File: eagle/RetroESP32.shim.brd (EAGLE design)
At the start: 56 x 34 mm, 2 parts

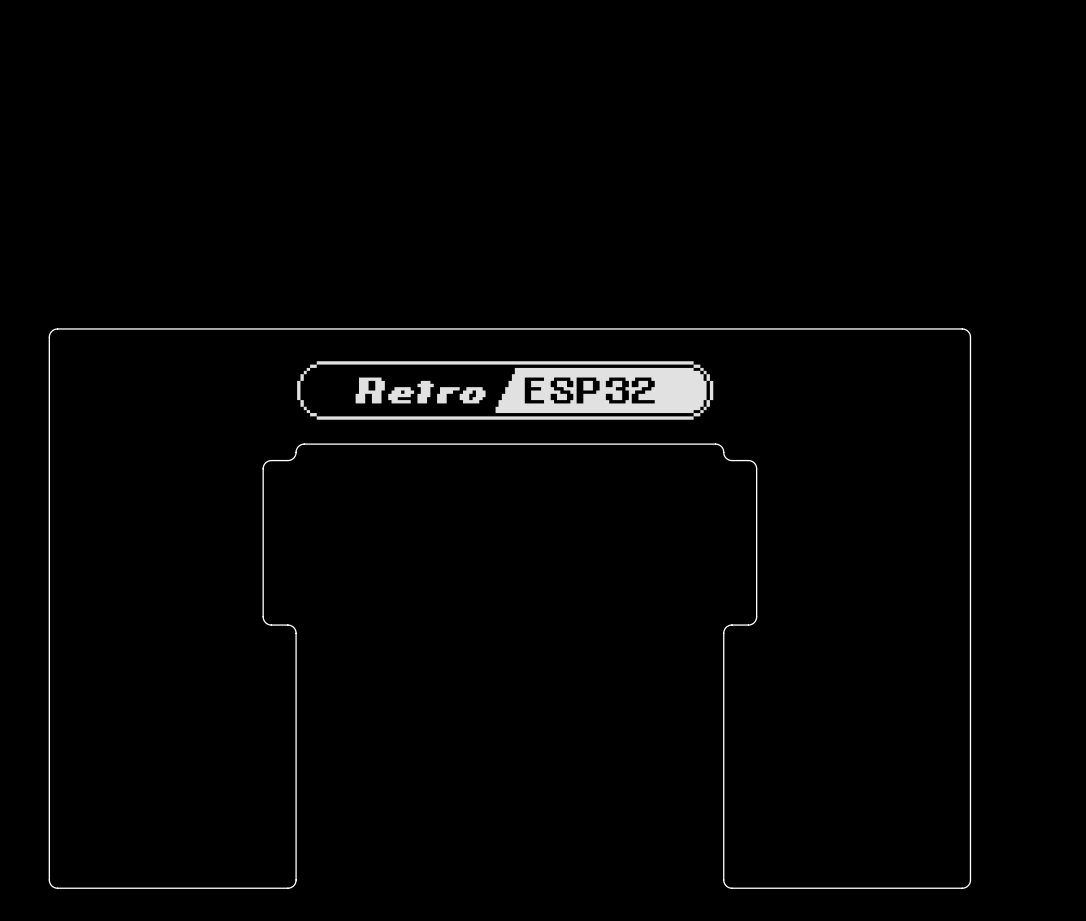
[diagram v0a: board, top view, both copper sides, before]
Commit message: feat: updated shim
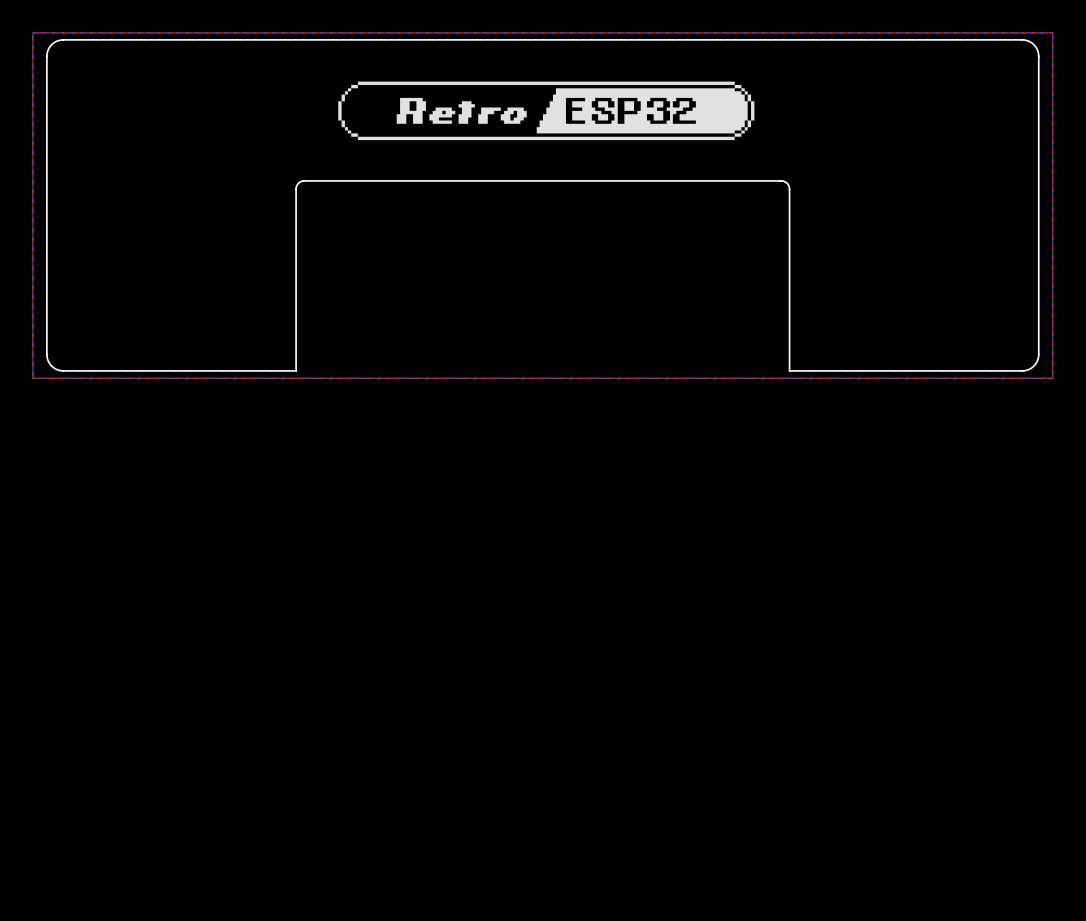
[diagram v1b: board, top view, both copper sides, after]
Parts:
- moved E$1 17.2 mm to (17.5, 49.0)
- moved U$1 17.1 mm to (38.5, 49.0)
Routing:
- added copper zone on layer 1, net GND
- added copper zone on layer 16, net GND
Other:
- board size 56 x 34 mm -> 60.3 x 20.1 mm
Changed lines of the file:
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@@
 <layer number="25" name="tNames" color="7" fill="1" visible="yes" active="yes"/>
 <layer number="26" name="bNames" color="7" fill="1" visible="yes" active="yes"/>
-<layer number="27" name="tValues" color="7" fill="1" visible="yes" active="yes"/>
-<layer number="28" name="bValues" color="7" fill="1" visible="yes" active="yes"/>
+<layer number="27" name="tValues" color="7" fill="1" visible="no" active="yes"/>
+<layer number="28" name="bValues" color="7" fill="1" visible="no" active="yes"/>
 <layer number="29" name="tStop" color="7" fill="3" visible="no" active="yes"/>
 <layer number="30" name="bStop" color="7" fill="6" visible="no" active="yes"/>
@@
 <layer number="41" name="tRestrict" color="4" fill="10" visible="yes" active="yes"/>
 <layer number="42" name="bRestrict" color="1" fill="10" visible="yes" active="yes"/>
-<layer number="43" name="vRestrict" color="2" fill="10" visible="yes" active="yes"/>
+<layer number="43" name="vRestrict" color="2" fill="10" visible="no" active="yes"/>
 <layer number="44" name="Drills" color="7" fill="1" visible="no" active="yes"/>
 <layer number="45" name="Holes" color="7" fill="1" visible="no" active="yes"/>
 <layer number="46" name="Milling" color="3" fill="1" visible="no" active="yes"/>
 <layer number="47" name="Measures" color="7" fill="1" visible="no" active="yes"/>
-<layer number="48" name="Document" color="7" fill="1" visible="yes" active="yes"/>
-<layer number="49" name="Reference" color="7" fill="1" visible="yes" active="yes"/>
+<layer number="48" name="Document" color="7" fill="1" visible="no" active="yes"/>
+<layer number="49" name="Reference" color="7" fill="1" visible="no" active="yes"/>
 <layer number="50" name="dxf" color="7" fill="1" visible="no" active="yes"/>
 <layer number="51" name="tDocu" color="7" fill="1" visible="yes" active="yes"/>
@@
 <board>
 <plain>
-<wire x1="0.5" y1="0" x2="14.5" y2="0" width="0" layer="20"/>
-<wire x1="14.5" y1="0" x2="15" y2="0.5" width="0" layer="20" curve="90"/>
-<wire x1="15" y1="0.5" x2="15" y2="15.5" width="0" layer="20"/>
-<wire x1="15" y1="15.5" x2="14.5" y2="16" width="0" layer="20" curve="90"/>
-<wire x1="15" y1="26.5" x2="15.5" y2="27" width="0" layer="20" curve="-90"/>
-<wire x1="15.5" y1="27" x2="40.5" y2="27" width="0" layer="20"/>
-<wire x1="40.5" y1="27" x2="41" y2="26.5" width="0" layer="20" curve="-90"/>
-<wire x1="41" y1="26.5" x2="41.5" y2="26" width="0" layer="20" curve="90"/>
-<wire x1="41.5" y1="26" x2="42.5" y2="26" width="0" layer="20"/>
-<wire x1="42.5" y1="26" x2="43" y2="25.5" width="0" layer="20" curve="-90"/>
-<wire x1="43" y1="25.5" x2="43" y2="16.5" width="0" layer="20"/>
-<wire x1="43" y1="16.5" x2="42.5" y2="16" width="0" layer="20" curve="-90"/>
-<wire x1="42.5" y1="16" x2="41.5" y2="16" width="0" layer="20"/>
-<wire x1="41.5" y1="16" x2="41" y2="15.5" width="0" layer="20" curve="90"/>
-<wire x1="41" y1="15.5" x2="41" y2="0.5" width="0" layer="20"/>
-<wire x1="41" y1="0.5" x2="41.5" y2="0" width="0" layer="20" curve="90"/>
-<wire x1="15" y1="26.5" x2="14.5" y2="26" width="0" layer="20" curve="-90"/>
-<wire x1="14.5" y1="26" x2="13.5" y2="26" width="0" layer="20"/>
-<wire x1="13.5" y1="26" x2="13" y2="25.5" width="0" layer="20" curve="90"/>
-<wire x1="13" y1="25.5" x2="13" y2="16.5" width="0" layer="20"/>
-<wire x1="13" y1="16.5" x2="13.5" y2="16" width="0" layer="20" curve="90"/>
-<wire x1="13.5" y1="16" x2="14.5" y2="16" width="0" layer="20"/>
-<wire x1="0.5" y1="0" x2="0" y2="0.5" width="0" layer="20" curve="-90"/>
-<wire x1="0" y1="0.5" x2="0" y2="33.5" width="0" layer="20"/>
-<wire x1="0" y1="33.5" x2="0.5" y2="34" width="0" layer="20" curve="-90"/>
-<wire x1="0.5" y1="34" x2="55.5" y2="34" width="0" layer="20"/>
-<wire x1="55.5" y1="34" x2="56" y2="33.5" width="0" layer="20" curve="-90"/>
-<wire x1="56" y1="33.5" x2="56" y2="0.5" width="0" layer="20"/>
-<wire x1="56" y1="0.5" x2="55.5" y2="0" width="0" layer="20" curve="-90"/>
-<wire x1="55.5" y1="0" x2="41.5" y2="0" width="0" layer="20"/>
+<wire x1="15" y1="31.45" x2="15" y2="42.5" width="0.1016" layer="20"/>
+<wire x1="15" y1="42.5" x2="15.5" y2="43" width="0.1016" layer="20" curve="-90"/>
+<wire x1="15.5" y1="43" x2="44.5" y2="43" width="0.1016" layer="20"/>
+<wire x1="44.5" y1="43" x2="45" y2="42.5" width="0.1016" layer="20" curve="-90"/>
+<wire x1="45" y1="42.5" x2="45" y2="31.45" width="0.1016" layer="20"/>
+<wire x1="59.15" y1="31.45" x2="45" y2="31.45" width="0.1016" layer="20"/>
+<wire x1="15" y1="31.45" x2="0.85" y2="31.45" width="0.1016" layer="20"/>
+<wire x1="0.85" y1="31.45" x2="-0.15" y2="32.45" width="0.1016" layer="20" curve="-90"/>
+<wire x1="-0.15" y1="32.45" x2="-0.15" y2="50.575" width="0.1016" layer="20"/>
+<wire x1="-0.15" y1="50.575" x2="0.85" y2="51.575" width="0.1016" layer="20" curve="-90"/>
+<wire x1="0.85" y1="51.575" x2="59.15" y2="51.575" width="0.1016" layer="20"/>
+<wire x1="59.15" y1="51.575" x2="60.15" y2="50.575" width="0.1016" layer="20" curve="-90"/>
+<wire x1="60.15" y1="50.575" x2="60.15" y2="32.45" width="0.1016" layer="20"/>
+<wire x1="60.15" y1="32.45" x2="59.15" y2="31.45" width="0.1016" layer="20" curve="-90"/>
 </plain>
 <attributes>
@@
 </autorouter>
 <elements>
-<element name="U$1" library="RetroESP32" library_urn="urn:adsk.eagle:library:12566846" package="GITHUB" package3d_urn="urn:adsk.eagle:package:12566909/2" value="GITHUB" x="37" y="32" smashed="yes" rot="MR0"/>
-<element name="E$1" library="RetroESP32" library_urn="urn:adsk.eagle:library:12566846" package="RETROESP32" package3d_urn="urn:adsk.eagle:package:12570035/2" value="" x="15" y="32" smashed="yes"/>
+<element name="U$1" library="RetroESP32" library_urn="urn:adsk.eagle:library:12566846" package="GITHUB" package3d_urn="urn:adsk.eagle:package:12566909/2" value="GITHUB" x="38.5" y="49" smashed="yes" rot="MR0"/>
+<element name="E$1" library="RetroESP32" library_urn="urn:adsk.eagle:library:12566846" package="RETROESP32" package3d_urn="urn:adsk.eagle:package:12570035/2" value="" x="17.5" y="49" smashed="yes"/>
 </elements>
 <signals>
+<signal name="GND">
+<polygon width="0.127" layer="16" thermals="no">
+<vertex x="-1" y="52"/>
+<vertex x="-1" y="31"/>
+<vertex x="61" y="31"/>
+<vertex x="61" y="52"/>
+</polygon>
+<polygon width="0.127" layer="1" thermals="no">
+<vertex x="-1" y="52"/>
+<vertex x="61" y="52"/>
+<vertex x="61" y="31"/>
+<vertex x="-1" y="31"/>
+</polygon>
+</signal>
 </signals>
 <mfgpreviewcolors>
